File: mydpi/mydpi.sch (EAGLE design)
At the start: 34 parts, among them Q1 DMN3404L, U1 MEGA32U4-MU, U2 RT9193-33GB, Y1 830069392

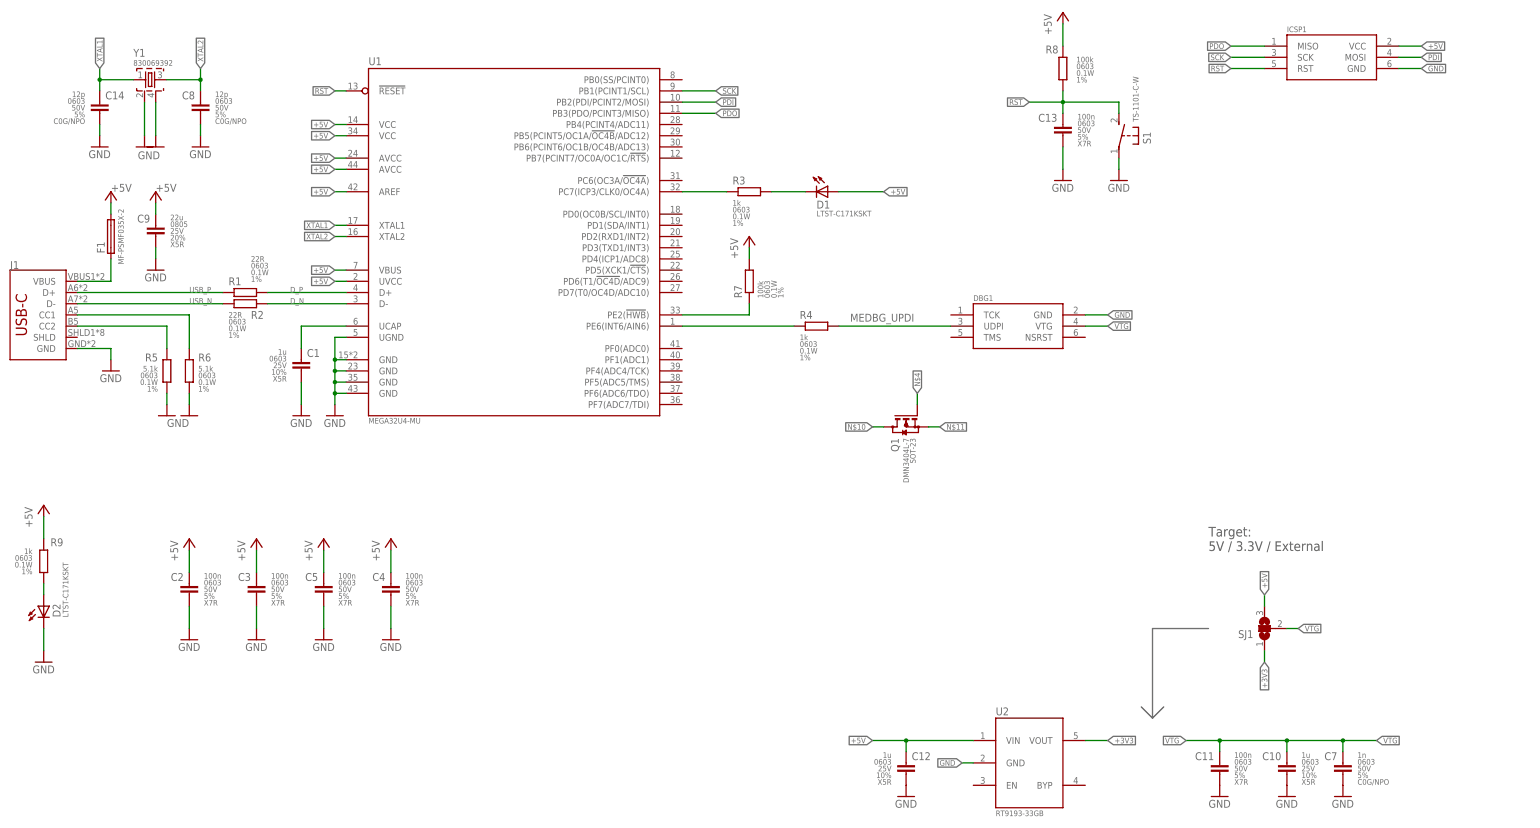
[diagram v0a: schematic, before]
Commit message: Bugfixes in used libraries
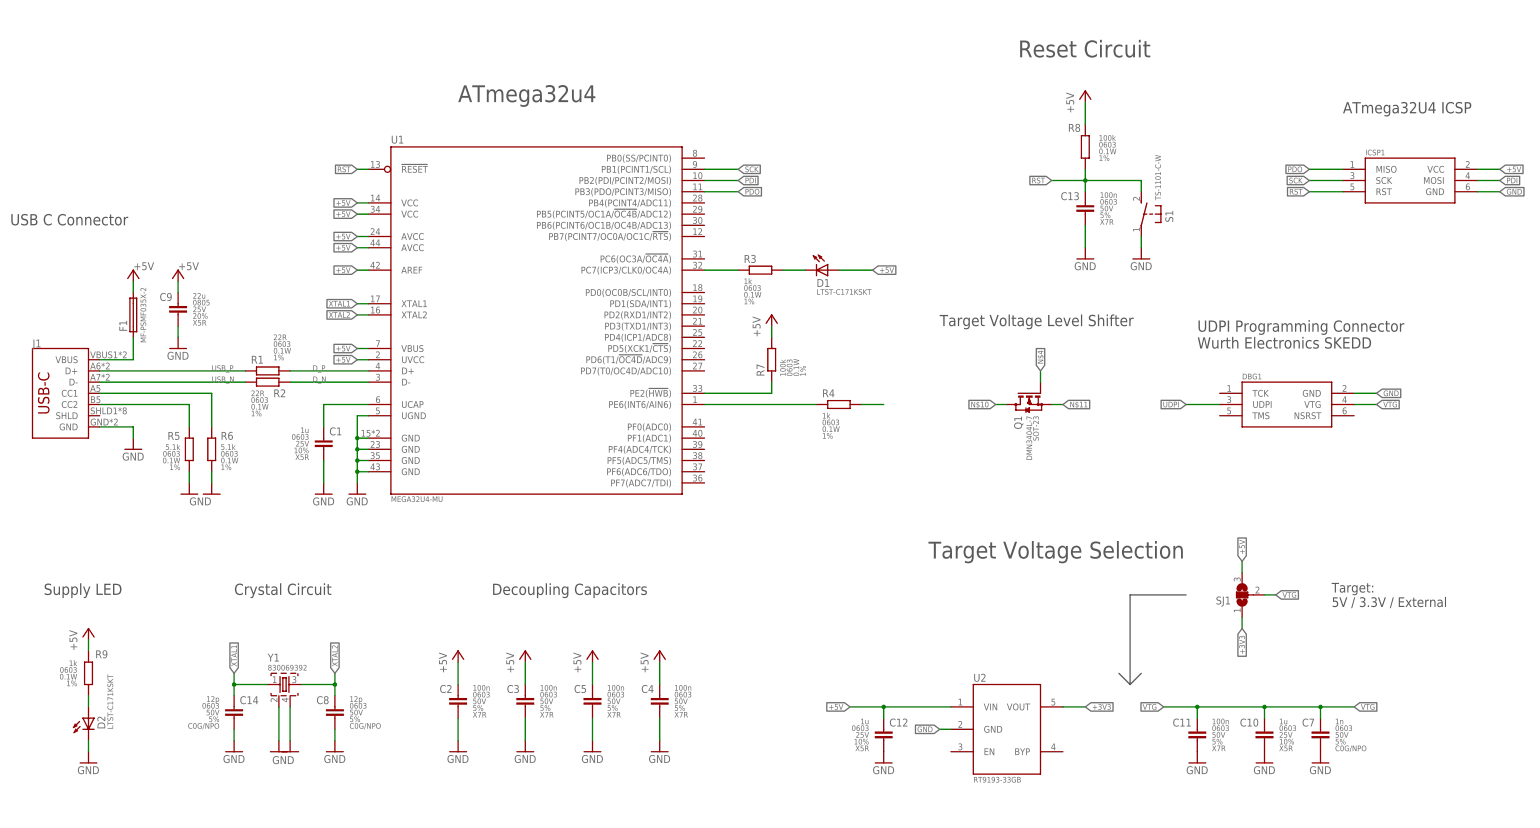
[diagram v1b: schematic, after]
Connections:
- removed net MEDBG_UPDI: DBG1.UDPI, R4.2
- new net N$3: R4.2
- new net UDPI: DBG1.UDPI
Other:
- note added: "ATmega32U4 ICSP"
- note added: "ATmega32u4"
- note added: "Crystal Circuit"
- note added: "Decoupling Capacitors"
- note added: "Reset Circuit"
- note added: "Supply LED"
- note added: "Target Voltage Level Shifter"
- note added: "Target Voltage Selection"
- note added: "UDPI Programming Connector Wurth Electronics SKEDD"
- note added: "USB C Connector"
- moved on the sheet: C1, C10, C11, C12, C13, C14, C2, C3, C4, C5, C7, C8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
